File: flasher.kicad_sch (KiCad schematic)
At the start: 22 parts, among them Q2 SS8050_C2150, Q3 SS8050_C2150, U5 CH343G

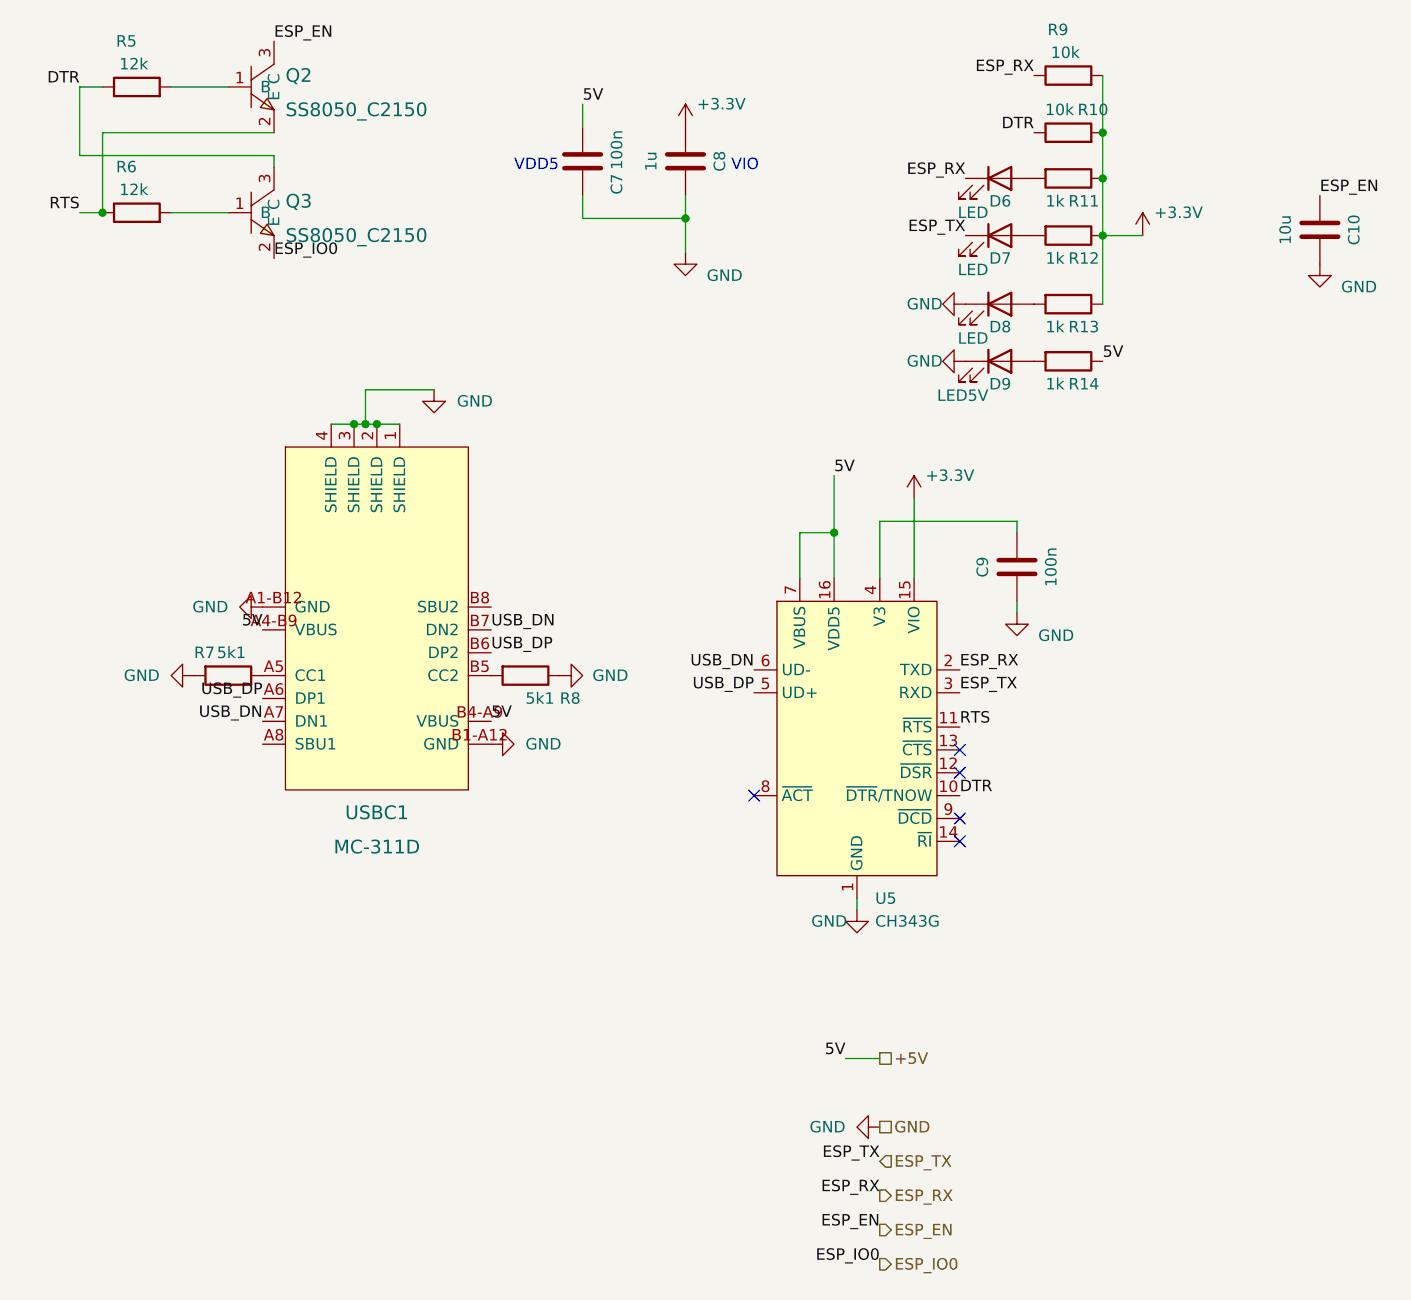
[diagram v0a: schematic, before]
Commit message: Weniger schwerbehinderte grid koordinaten
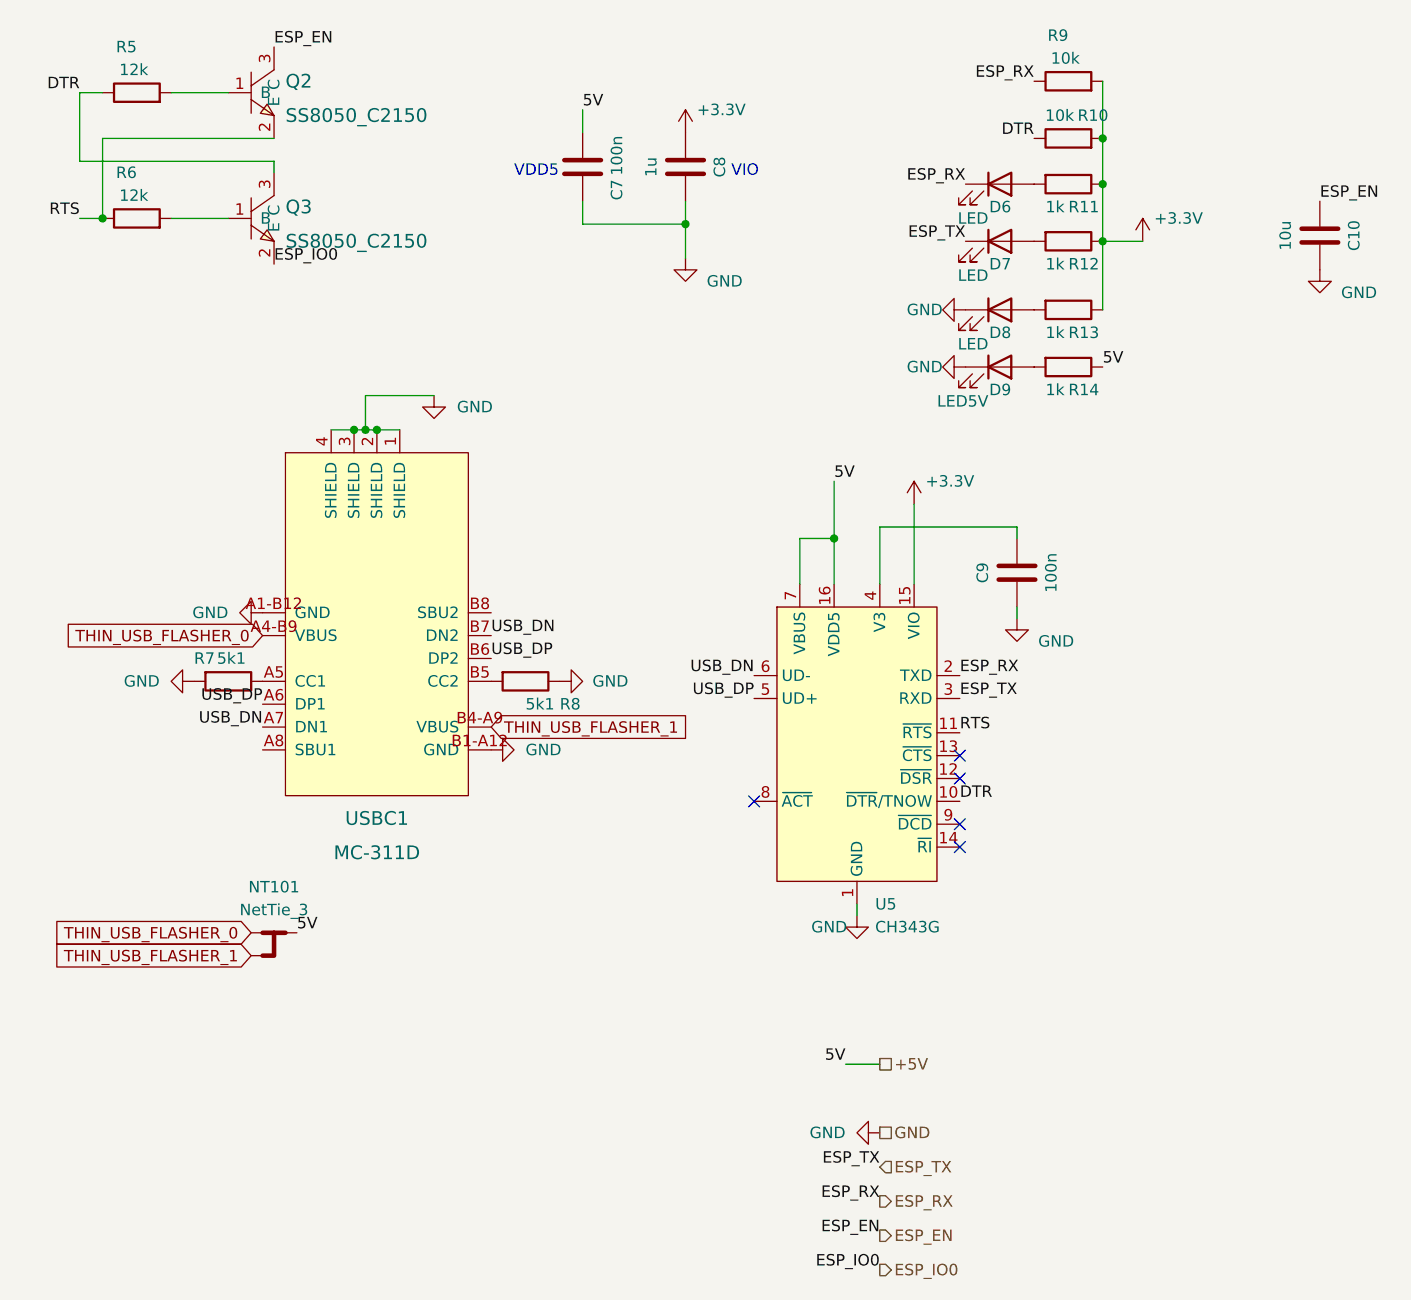
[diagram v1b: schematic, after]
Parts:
- added NT101: NetTie_3, NetTie:NetTie-3_SMD_Pad0.5mm, symbol Device:NetTie_3
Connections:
- net +5V: now also NT101.2; no longer USBC1.A4-B9 (VBUS), USBC1.B4-A9 (VBUS)
- new net THIN_USB_FLASHER_0: NT101.1, USBC1.A4-B9 (VBUS)
- new net THIN_USB_FLASHER_1: NT101.3, USBC1.B4-A9 (VBUS)
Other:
- moved on the sheet: C10, C7, C8, C9, D6, D7, D8, D9, Q2, Q3, R10, R11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
